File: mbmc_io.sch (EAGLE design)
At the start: 49 parts, among them IC1 PIC18F47Q84-E_P, IC2 7805TV, U1 REF3440IDBVR, U2 TCAN330GDR, X1 GLX-S-88M

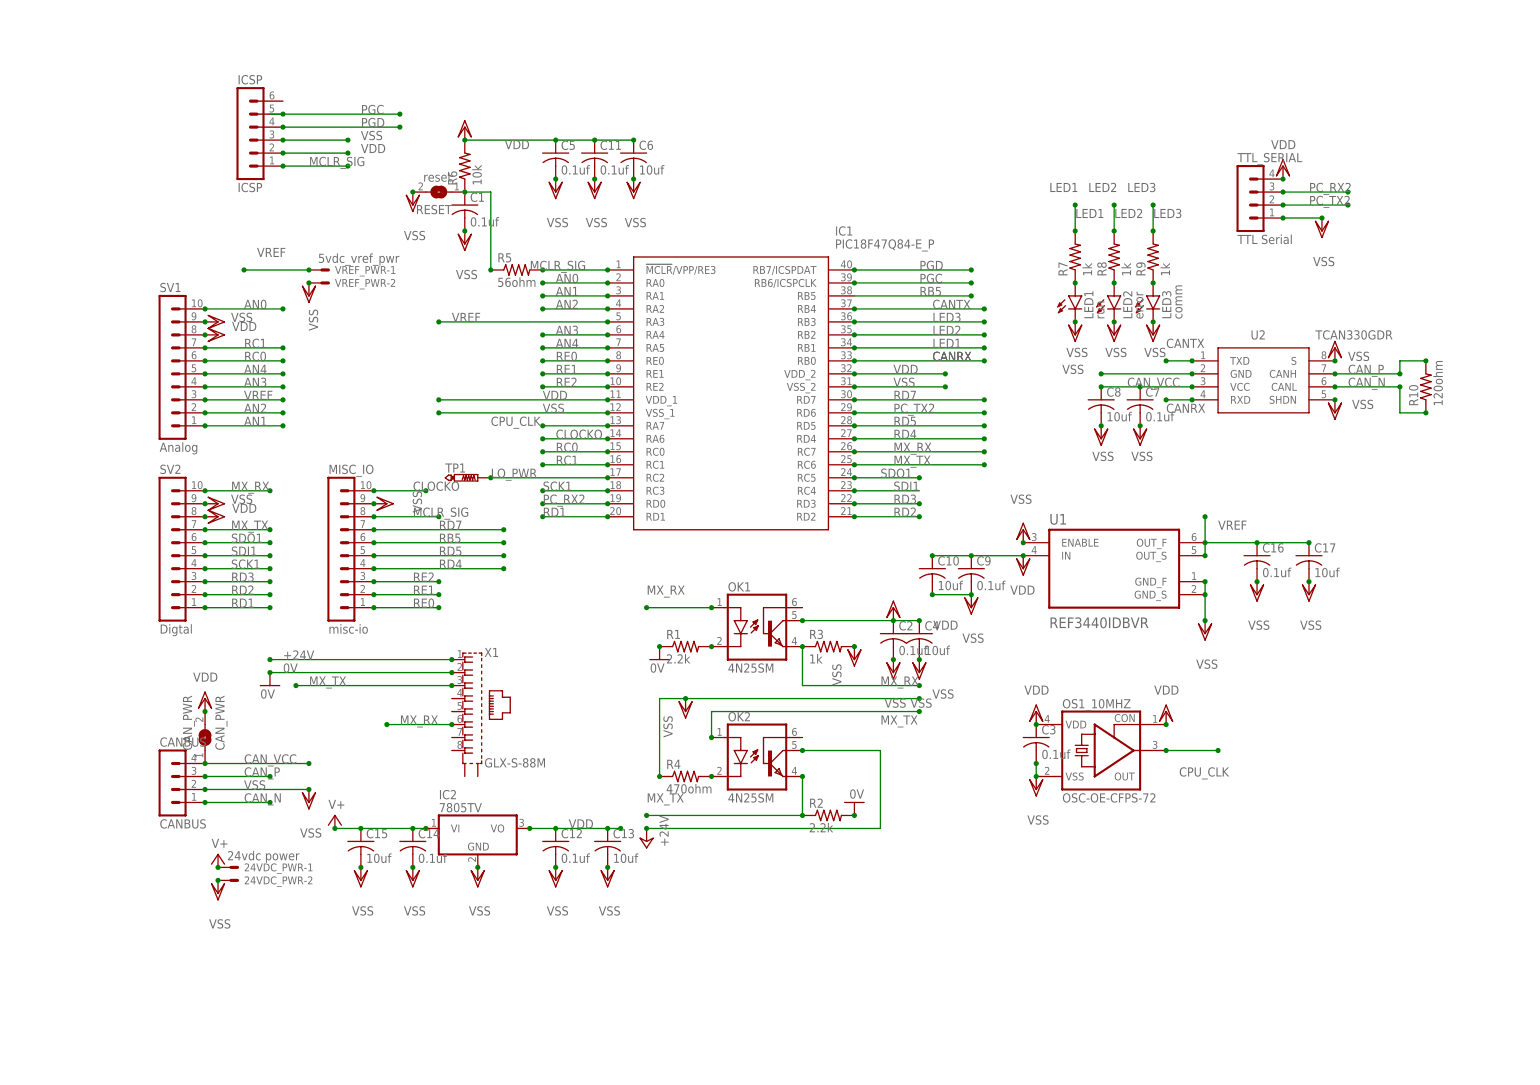
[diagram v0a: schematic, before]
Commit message: up
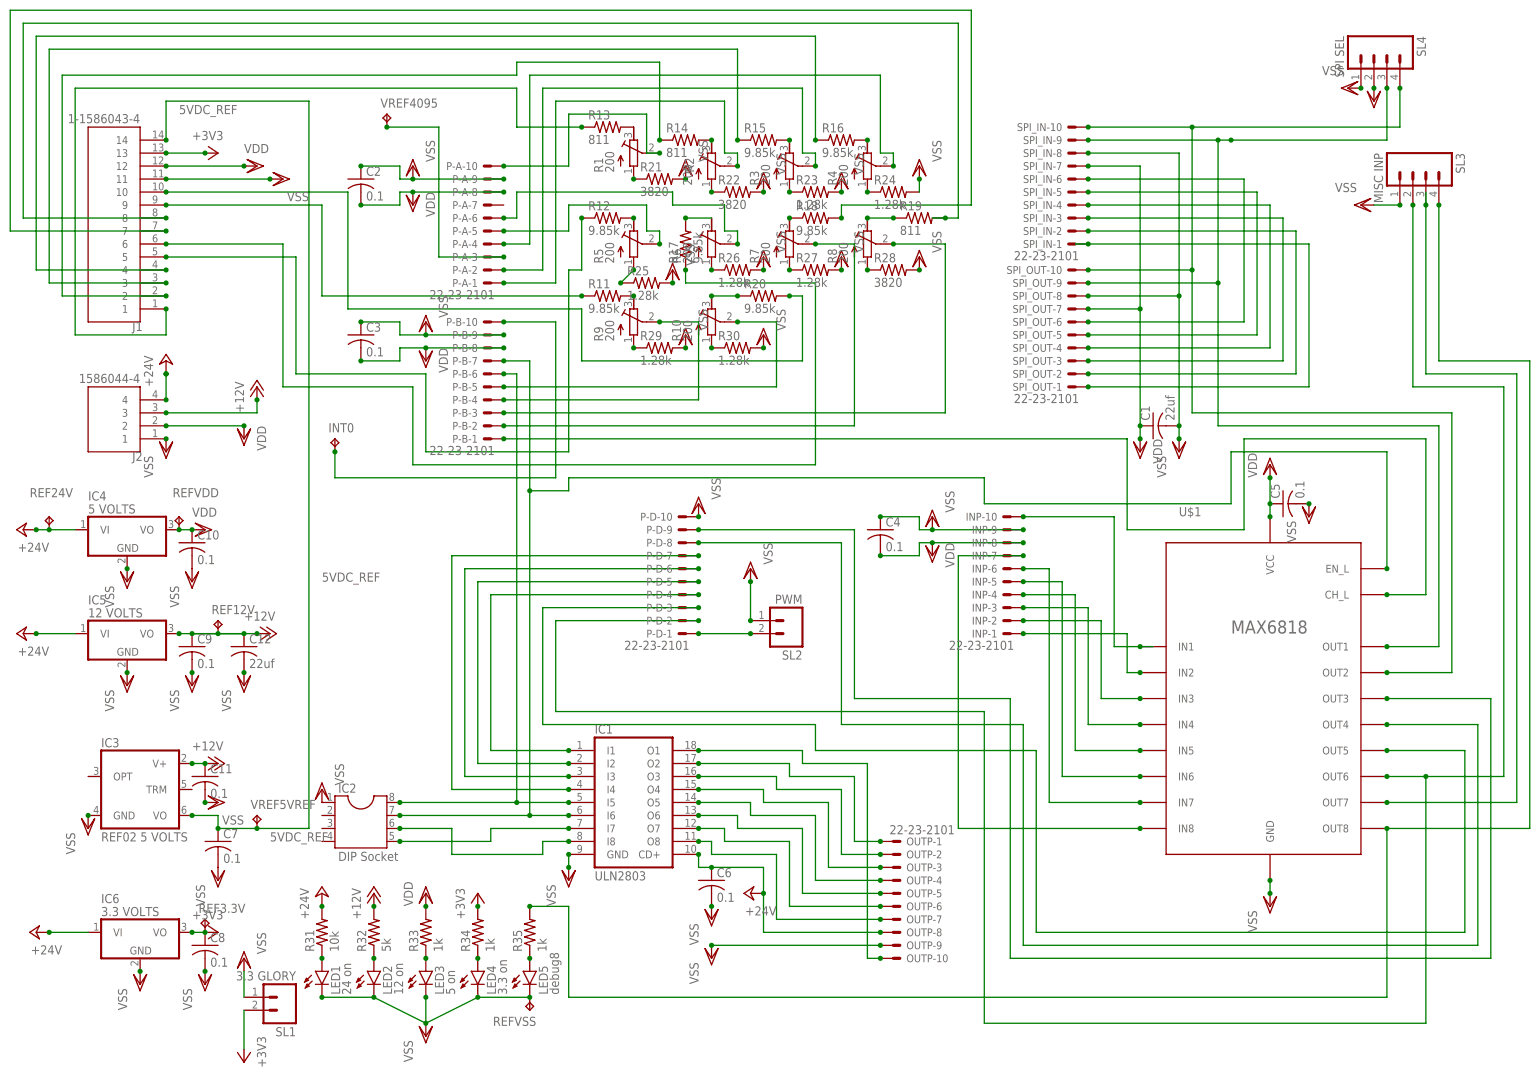
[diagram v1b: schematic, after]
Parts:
- removed 24VDC_PWR: 24vdc power, con-molex:22-23-2021
- removed C13, C15, C17: 10uf, rcl:C-USC0805
- removed C14, C16: 0.1uf, rcl:C-USC0805
- removed CANBUS: CANBUS, con-lstb:MA04-1
- removed CAN_PWR: CAN_PWR, jumper:SJ
- removed ICSP: ICSP, con-lstb:MA06-1
- removed MISC_IO: misc-io, con-lstb:MA10-1
- removed OK1, OK2: 4N25SM, optocoupler:4N25SM
- removed OS1_10MHZ: OSC-OE-CFPS-72, IQD-Frequency-Products:OSC-OE-CFPS-72
- removed RESET: reset, jumper:SJ
- removed SV1: Analog, con-lstb:MA10-1
- removed SV2: Digtal, con-lstb:MA10-1
- removed TP1: PTR1PAD1-13, testpad:PTR1PAD1-13
- removed TTL_SERIAL: TTL Serial, con-lstb:MA04-1
- removed U1: REF3440IDBVR, REF3440IDBVR:REF3440IDBVR
- removed U2: TCAN330GDR, TCAN330GDR:TCAN330GDR
- removed VREF_PWR: 5vdc_vref_pwr, con-molex:22-23-2021
- removed X1: GLX-S-88M, con-kycon:GLX-S-88M
- added IC3: REF02 5 VOLTS, linear:REF02Z
- added IC4: 5 VOLTS, linear:7805TV
- added IC5: 12 VOLTS, linear:7805TV
- added IC6: 3.3 VOLTS, linear:7805TV
- added INP, OUTP, P-A, P-B, P-D, SPI_IN, SPI_OUT: 22-23-2101, con-molex:22-23-2101
- added INT0, REF12V, REF24V, REF3.3V, REFVDD, REFVSS, VREF4095, VREF5VREF: TPB1,27, testpad:TPB1,27
- added J1: 1-1586043-4, 1-1586043-4:1-1586043-4
- added J2: 1586044-4, 1586044-4:1586044-4
- added LED4: 3.3 on, led:LEDCHIPLED_1206
- added LED5: debug8, led:LEDCHIPLED_1206
- added R11, R12, R15, R16, R17, R18, R20: 9.85k, rcl:R-US_R0805
- added R13, R14, R19: 811, rcl:R-US_R0805
- added R21, R22, R28: 3820, rcl:R-US_R0805
- added R23, R24, R25, R26, R27, R29, R30: 1.28k, rcl:R-US_R0805
- added R31: 10k, rcl:R-US_R0805
- added R32: 5k, rcl:R-US_R0805
- added R33, R34, R35: 1k, rcl:R-US_R0805
- added SL1: 3.3 GLORY, con-amp-quick:M02
- added SL2: PWM, con-amp-quick:M02
- added SL3: MISC INP, con-amp-quick:M04
- added SL4: SPI SEL, con-amp-quick:M04
- added U$1: MAX6818, MAX6818:MAX6818
- C1, C12: value 0.1uf -> 22uf
- C10, C4, C6, C8: value 10uf -> 0.1
- C11, C2, C3, C5, C7, C9: value 0.1uf -> 0.1
- IC1: value PIC18F47Q84-E_P -> ULN2803; device PIC18F47Q84-E_P:PIC18F47Q84-E_P -> uln-udn:ULN2803A
- IC2: value 7805TV -> DIP Socket; device linear:7805TV -> ic-package:DIL8S
- LED1: value run -> 24 on; device led:LEDCHIPLED_0805 -> led:LEDCHIPLED_1206
- LED2: value error -> 12 on; device led:LEDCHIPLED_0805 -> led:LEDCHIPLED_1206
- LED3: value comm -> 5 on; device led:LEDCHIPLED_0805 -> led:LEDCHIPLED_1206
- R1, R2: value 2.2k -> 200; device rcl:R-US_R0805 -> rcl:R-TRIMM3339P
- R10: value 120ohm -> 200; device rcl:R-US_R0805 -> rcl:R-TRIMM3339P
- R3, R7, R8, R9: value 1k -> 200; device rcl:R-US_R0805 -> rcl:R-TRIMM3339P
- R4: value 470ohm -> 200; device rcl:R-US_R0805 -> rcl:R-TRIMM3339P
- R5: value 56ohm -> 200; device rcl:R-US_R0805 -> rcl:R-TRIMM3339P
- R6: value 10k -> 200; device rcl:R-US_R0805 -> rcl:R-TRIMM3339P
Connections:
- removed net 0V: R1.1, R2.2, X1.2
- removed net AN0: IC1.RA0, SV1.10
- removed net AN1: IC1.RA1, SV1.1
- removed net AN2: IC1.RA2, SV1.2
- removed net AN3: IC1.RA4, SV1.4
- removed net AN4: IC1.RA5, SV1.5
- removed net CANRX: IC1.RB0, U2.RXD
- removed net CANTX: IC1.RB4, U2.TXD
- removed net CAN_N: CANBUS.1, R10.1, U2.CANL
- removed net CAN_P: CANBUS.3, R10.2, U2.CANH
- removed net CAN_VCC: C7.1, C8.1, CANBUS.4, CAN_PWR.1, U2.VCC
- removed net CLOCKO: IC1.RA6, MISC_IO.10
- removed net CPU_CLK: IC1.RA7, OS1_10MHZ.OUT
- removed net LED1: IC1.RB1, R7.2
- removed net LED2: IC1.RB2, R8.2
- removed net LED3: IC1.RB3, R9.2
- removed net LO_PWR: IC1.RC2, TP1.TP
- removed net MCLR_SIG: IC1.!MCLR!/VPP/RE3, ICSP.1, MISC_IO.8, R5.2
- removed net MX_RX: IC1.RC7, OK1.A, OK1.EMI, R3.1, SV2.10, X1.6
- removed net MX_TX: IC1.RC6, OK2.A, OK2.EMI, R2.1, SV2.7, X1.3
- removed net PC_RX2: IC1.RD0, TTL_SERIAL.3
- removed net PC_TX2: IC1.RD6, TTL_SERIAL.2
- removed net PGC: IC1.RB6/ICSPCLK, ICSP.5
- removed net PGD: IC1.RB7/ICSPDAT, ICSP.4
- removed net RB5: IC1.RB5, MISC_IO.6
- removed net RC0: IC1.RC0, SV1.6
- removed net RC1: IC1.RC1, SV1.7
- removed net RD1: IC1.RD1, SV2.1
- removed net RD2: IC1.RD2, SV2.2
- removed net RD3: IC1.RD3, SV2.3
- removed net RD4: IC1.RD4, MISC_IO.4
- removed net RD5: IC1.RD5, MISC_IO.5
- removed net RD7: IC1.RD7, MISC_IO.7
- removed net RE0: IC1.RE0, MISC_IO.1
- removed net RE1: IC1.RE1, MISC_IO.2
- removed net RE2: IC1.RE2, MISC_IO.3
- removed net SCK1: IC1.RC3, SV2.4
- removed net SDI1: IC1.RC4, SV2.5
- removed net SDO1: IC1.RC5, SV2.6
- removed net V+: 24VDC_PWR-1.S, C14.1, C15.1, IC2.VI
- removed net VREF: C16.1, C17.1, IC1.RA3, SV1.3, U1.OUT_F, U1.OUT_S, VREF_PWR-1.S
- new net +12V: C11.1, C12.1, C9.1, IC3.V+, IC5.VO, J2.3, R32.2, REF12V.TP
- new net +3V3: C8.1, IC6.VO, J1.13, R34.2, REF3.3V.TP, SL1.2
- new net 5VDC_REF: C7.1, IC3.VO, J1.14, VREF5VREF.TP
- new net N$10: J1.8, R19.2
- new net N$11: R1.A, R21.1
- new net N$12: R2.A, R22.1
- new net N$13: R23.1, R3.A
- new net N$14: R24.1, R4.A
- new net N$15: R25.1, R5.A
- new net N$16: R26.1, R6.A
- new net N$17: R27.1, R7.A
- new net N$18: R28.1, R8.A
- new net N$19: R29.1, R9.A
- new net N$20: R10.A, R30.1
- new net N$21: P-A-10.S, R1.S
- new net N$22: P-A-1.S, R2.S
- new net N$23: P-A-2.S, R3.S
- new net N$24: J1.2, R14.1
- new net N$25: P-A-5.S, R5.S
- new net N$26: P-A-6.S, R6.S
- new net N$27: P-B-2.S, R7.S
- new net N$28: P-B-3.S, R8.S
- new net N$29: P-B-4.S, R9.S
- new net N$30: P-B-5.S, R10.S
- new net N$31: IC1.I1, P-D-4.S
- new net N$32: IC1.I2, P-D-5.S
- new net N$33: IC1.I3, P-D-6.S
- new net N$34: IC1.I4, P-D-7.S
- new net N$35: IC1.I5, IC2.8, P-B-6.S
- new net N$36: IC1.I6, IC2.7, P-B-7.S, U$1.EN_L
- new net N$37: IC1.I7, IC2.5
- new net N$38: IC1.I8, IC2.6
- new net N$39: SL4.3, SPI_IN-9.S, SPI_OUT-9.S, U$1.OUT1
- new net N$40: P-B-1.S, U$1.CH_L
- new net N$41: P-D-9.S, U$1.OUT3
- new net N$42: P-D-8.S, U$1.OUT4
- new net N$43: P-D-3.S, U$1.OUT5
- new net N$44: INP-10.S, U$1.IN1
- new net N$45: SL4.4, SPI_IN-10.S, SPI_OUT-10.S, U$1.OUT2
- new net N$46: INP-1.S, U$1.IN2
- new net N$47: INP-2.S, U$1.IN3
- new net N$48: INP-3.S, U$1.IN4
- new net N$49: INP-4.S, U$1.IN5
- new net N$50: INP-5.S, U$1.IN6
- new net N$51: INP-6.S, U$1.IN7
- new net N$52: INP-7.S, U$1.IN8
- new net N$53: IC1.O1, OUTP-10.S
- new net N$54: IC1.O2, OUTP-1.S
- new net N$55: IC1.O3, OUTP-2.S
- new net N$56: IC1.O4, OUTP-3.S
- new net N$57: IC1.O5, OUTP-4.S
- new net N$58: IC1.O6, OUTP-5.S
- new net N$59: IC1.O7, OUTP-6.S
- new net N$60: IC1.O8, OUTP-7.S
- new net N$62: SPI_IN-6.S, SPI_OUT-6.S
- new net N$63: SPI_IN-5.S, SPI_OUT-5.S
- new net N$64: SPI_IN-4.S, SPI_OUT-4.S
- new net N$65: SPI_IN-3.S, SPI_OUT-3.S
- new net N$66: SPI_IN-2.S, SPI_OUT-2.S
- new net N$67: SPI_IN-1.S, SPI_OUT-1.S
- new net N$68: J1.4, R16.1
- new net N$69: J1.9, R11.1
- new net N$7: R17.2, R6.E
- new net N$70: J1.3, R15.1
- new net N$71: J1.10, R20.2
- new net N$72: J1.5, R12.1
- new net N$73: J1.6, R17.1
- new net N$74: J1.1, R13.1
- new net N$75: P-A-4.S, R4.S
- new net N$76: LED1.A, R31.1
- new net N$77: LED2.A, R32.1
- new net N$78: LED3.A, R33.1
- new net N$79: LED4.A, R34.1
- new net N$8: J1.7, R18.2
- new net N$80: LED5.A, R35.1
- new net N$81: R35.2, SL3.4, U$1.OUT8
- new net N$82: P-D-1.S, SL2.2
- new net N$83: R10.E, R20.1
- new net N$84: SL3.3, U$1.OUT7
- new net N$85: P-A-3.S, VREF4095.TP
- new net N$86: P-D-2.S, SL3.2, U$1.OUT6
- new net N$87: INT0.TP, P-B-10.S
- new net N$88: R18.1, R7.E
- new net N$9: R19.1, R8.E
- net +24V: now also C6.1, IC1.CD+, IC4.VI, IC5.VI, IC6.VI, J2.4, OUTP-8.S, R31.2, REF24V.TP; no longer OK2.COL, X1.1
- net N$1: now also R11.2, R9.E; no longer OK1.C, R1.2
- net N$2: now also R12.2, R5.E; no longer C1.1, R5.1, R6.1, RESET.1
- net N$3: now also R1.E, R13.2; no longer OK2.C, R4.2
- net N$4: now also R14.2, R2.E; no longer LED1.A, R7.1
- net N$5: now also R15.2, R3.E; no longer LED2.A, R8.1
- net N$6: now also R16.2, R4.E; no longer LED3.A, R9.1
- net VDD: now also C1.1, C2.2, C3.2, C4.2, IC4.VO, INP-8.S, J1.12, J2.2, P-A-8.S, P-B-8.S, R33.2, REFVDD.TP, SL4.2, SPI_IN-7.S, SPI_OUT-7.S, U$1.VCC; no longer C11.1, C12.1, C13.1, C2.1, C3.1, C4.1, C6.1, C9.1, CAN_PWR.2, IC1.VDD_1, IC1.VDD_2, IC2.VO, ICSP.2, OK1.COL, OS1_10MHZ.CON, OS1_10MHZ.VDD, R6.2, SV1.8, SV2.8, TTL_SERIAL.4, U1.IN
- net VSS: now also C2.1, C3.1, C4.1, IC1.GND, IC2.1, IC3.GND, IC4.GND, IC5.GND, IC6.GND, INP-9.S, J1.11, J2.1, LED4.C, LED5.C, OUTP-9.S, P-A-9.S, P-B-9.S, P-D-10.S, R21.2, R22.2, R23.2, R24.2, R25.2, R26.2, R27.2, R28.2, R29.2, R30.2, REFVSS.TP, SL1.1, SL2.1, SL3.1, SL4.1, SPI_IN-8.S, SPI_OUT-8.S, U$1.GND; no longer 24VDC_PWR-2.S, C13.2, C14.2, C15.2, C16.2, C17.2, C2.2, C3.2, C4.2, CANBUS.2, IC1.VSS_1, IC1.VSS_2, IC2.GND, ICSP.3, MISC_IO.9, OS1_10MHZ.VSS, R3.2, R4.1, RESET.2, SV1.9, SV2.9, TTL_SERIAL.1, U1.ENABLE, U1.GND_F, U1.GND_S, U2.GND, U2.S, U2.SHDN, VREF_PWR-2.S
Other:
- moved on the sheet: C1, C10, C11, C12, C2, C3, C4, C5, C6, C7, C8, C9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
